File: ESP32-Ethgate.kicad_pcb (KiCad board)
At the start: 2 copper layers, 71.2 x 38.1 mm, 56 parts, among them J1 USB_B_Micro, J2 HR911105A, J3 USB, J4 GPIO, Q1 UMH3N, U1 HT7233, U2 ESP32-WROOM-32U, U3 CH340C, U4 HT7233, U5 LAN8720A, U6 USBLC6-2SC6

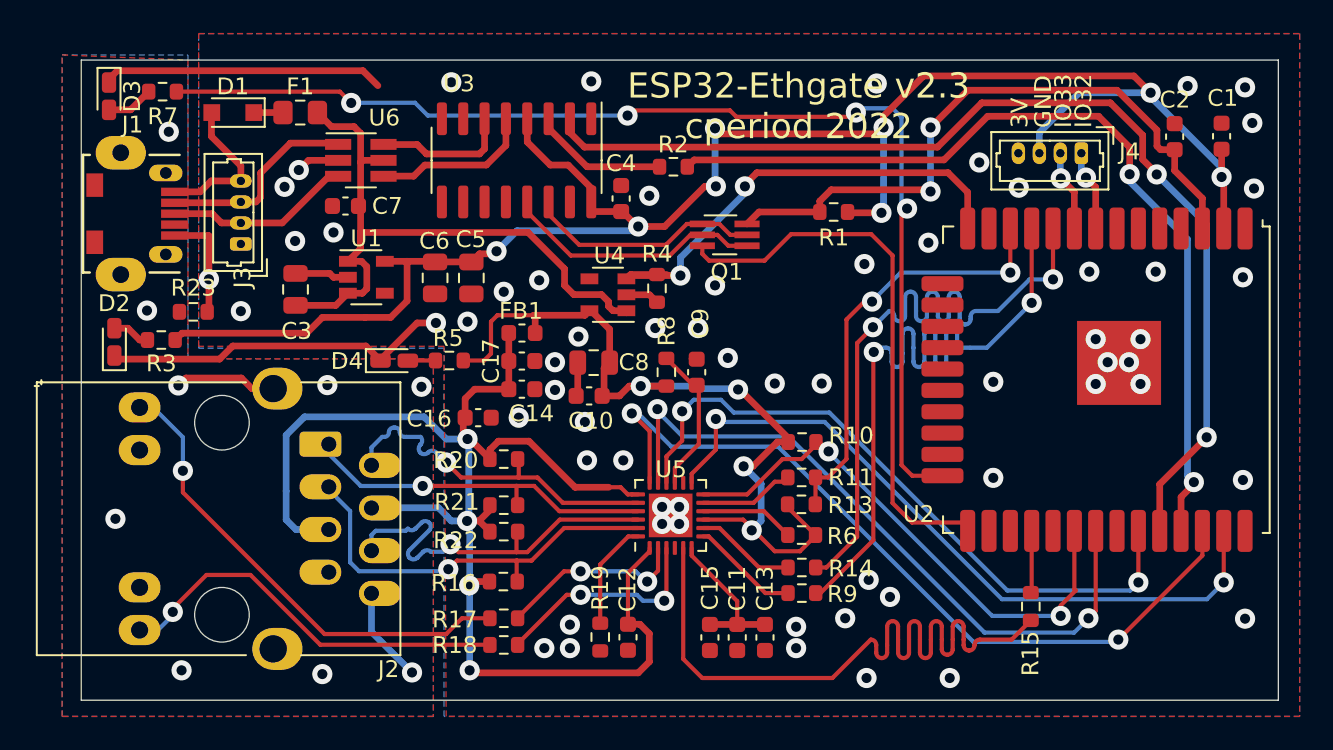
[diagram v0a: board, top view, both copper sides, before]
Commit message: update the various extra files
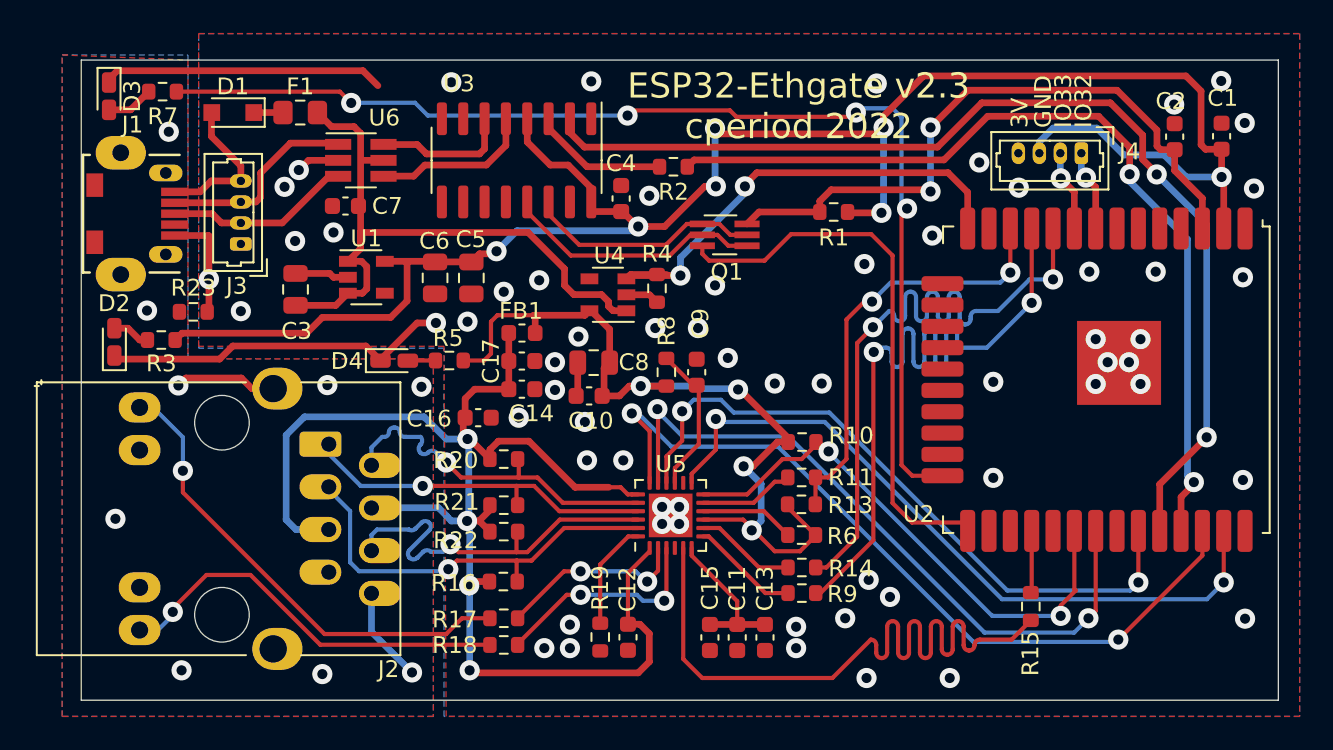
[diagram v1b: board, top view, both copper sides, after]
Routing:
- net +3V3: track 110.1 -> 113.5 mm, vias 8 -> 7
- net Net-(J2-Pad12): track 24.2 -> 23.1 mm
- net +3.3VA: track 84.9 -> 84.0 mm
- net /+3V3_LAN: track 49.8 -> 49.0 mm
- net Net-(J2-Pad9): track 28.8 -> 27.9 mm
- net RTS: track 14.1 -> 13.3 mm
- net /TX+: track 21.6 -> 20.9 mm
- net DTR: track 15.5 -> 14.9 mm
- net Net-(R2-Pad2): track 8.12 -> 7.55 mm
- net /DP: track 11.1 -> 10.6 mm
